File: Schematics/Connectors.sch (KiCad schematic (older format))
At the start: 130 parts, among them P501 CONN_02X05, P502 CONN_02X05, P503 CONN_02X05, P504 CONN_02X05, P505 CONN_6X2, P506 CONN_02X20, P507 CONN_02X05, P508 CONN_02X05, P509 CONN_02X05, P510 CONN_02X05, P511 CONN_02X05, P512 CONN_02X05, P513 CONN_02X05, P514 CONN_02X05, P515 CONN_02X05, P516 CONN_02X05, U501 NB3L553, U502 NB3L553

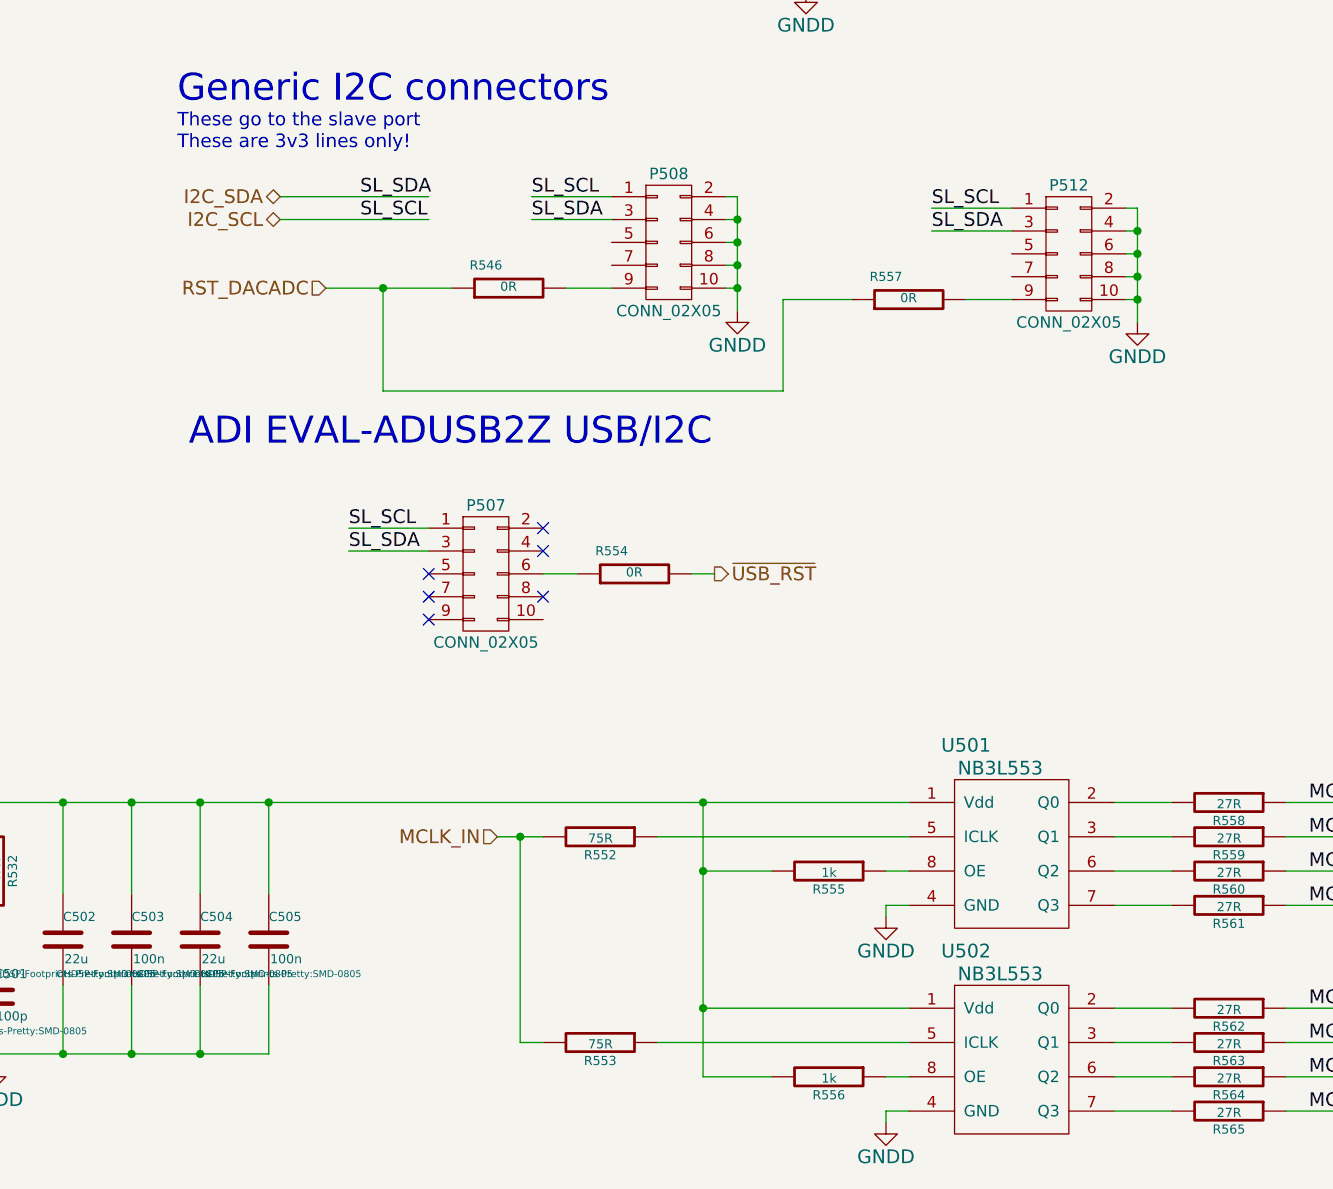
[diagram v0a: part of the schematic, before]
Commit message: WIP
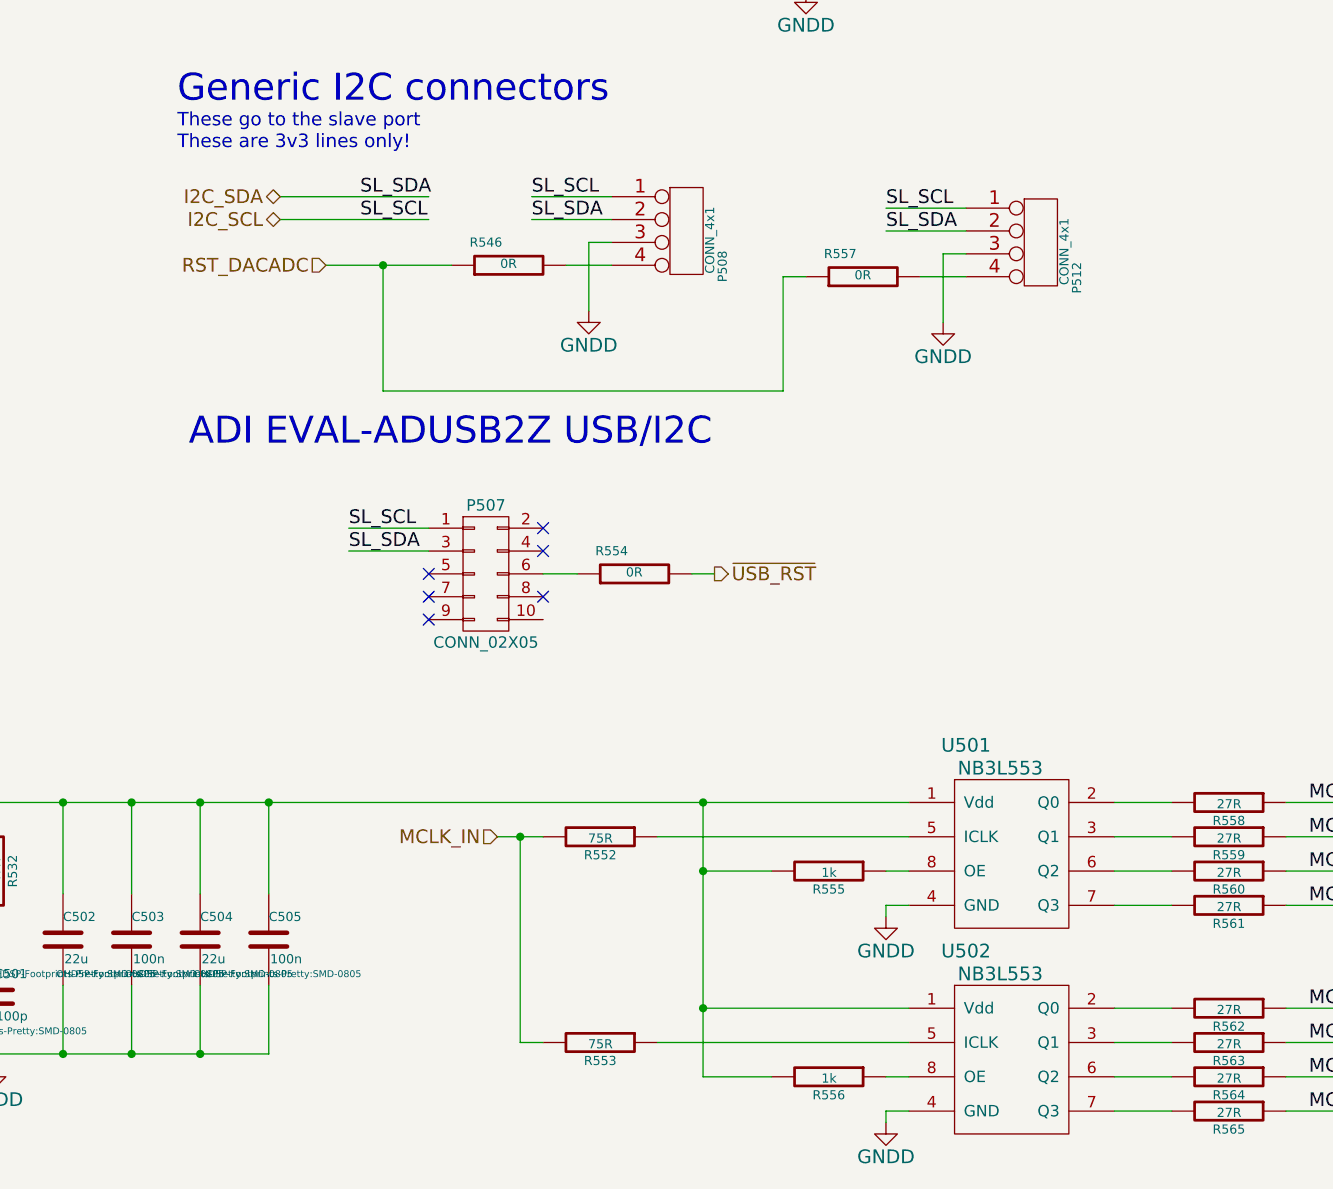
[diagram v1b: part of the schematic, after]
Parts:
- removed P508, P512: CONN_02X05, OHDSP-Footprints-Pretty:CONN_DIL_2X5, symbol CONN_02X05
- added P508, P512: CONN_4x1, OHDSP-Footprints-Pretty:CONN_SIL_4, symbol CONN_4x1
- P507: footprint OHDSP-Footprints-Pretty:CONN_DIL_2X5 -> OHDSP-Footprints-Pretty:CONN_DIL_2X5_BOX
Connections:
- wire segments 465 -> 457
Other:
- moved on the sheet: R546, R557
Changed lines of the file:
@@
 	1    0    0    -1
 $EndComp
-$Comp
-L CONN_02X05 P507
-U 1 1 54DC056C
-P 7400 8550
-F 0 "P507" H 7400 8850 50  0000 C CNN
-F 1 "CONN_02X05" H 7400 8250 50  0000 C CNN
-F 2 "OHDSP-Footprints-Pretty:CONN_DIL_2X5" H 7400 7350 60  0001 C CNN
-F 3 "" H 7400 7350 60  0000 C CNN
-	1    7400 8550
-	1    0    0    -1
-$EndComp
 Text Notes 6100 8000 0    118  ~ 0
 ADI EVAL-ADUSB2Z USB/I2C
@@
 L GNDD #PWR091
 U 1 1 54DC2149
-P 8500 7400
-F 0 "#PWR091" H 8500 7150 60  0001 C CNN
-F 1 "GNDD" H 8500 7250 60  0000 C CNN
-F 2 "" H 8500 7400 60  0000 C CNN
-F 3 "" H 8500 7400 60  0000 C CNN
-	1    8500 7400
+P 7850 7400
+F 0 "#PWR091" H 7850 7150 60  0001 C CNN
+F 1 "GNDD" H 7850 7250 60  0000 C CNN
+F 2 "" H 7850 7400 60  0000 C CNN
+F 3 "" H 7850 7400 60  0000 C CNN
+	1    7850 7400
 	1    0    0    -1
 $EndComp
@@
 $EndComp
 $Comp
-L CONN_02X05 P508
-U 1 1 54E480C2
-P 8200 7100
-F 0 "P508" H 8200 7400 50  0000 C CNN
-F 1 "CONN_02X05" H 8200 6800 50  0000 C CNN
-F 2 "OHDSP-Footprints-Pretty:CONN_DIL_2X5" H 8200 5900 60  0001 C CNN
-F 3 "" H 8200 5900 60  0000 C CNN
-	1    8200 7100
-	1    0    0    -1
-$EndComp
-$Comp
 L R R538
 U 1 1 54E4AF9E
@@
 $EndComp
 $Comp
-L CONN_02X05 P512
-U 1 1 54E55D44
-P 9950 7150
-F 0 "P512" H 9950 7450 50  0000 C CNN
-F 1 "CONN_02X05" H 9950 6850 50  0000 C CNN
-F 2 "OHDSP-Footprints-Pretty:CONN_DIL_2X5" H 9950 5950 60  0001 C CNN
-F 3 "" H 9950 5950 60  0000 C CNN
-	1    9950 7150
-	1    0    0    -1
-$EndComp
-$Comp
 L DIODE D501
 U 1 1 54E4E268
@@
 Text Label 7600 7000 0    60   ~ 0
 SL_SDA
-Text Label 9350 6950 0    60   ~ 0
-SL_SCL
-Text Label 9350 7050 0    60   ~ 0
-SL_SDA
-$Comp
-L GNDD #PWR0124
-U 1 1 551A75F1
-P 10250 7450
-F 0 "#PWR0124" H 10250 7200 60  0001 C CNN
-F 1 "GNDD" H 10250 7300 60  0000 C CNN
-F 2 "" H 10250 7450 60  0000 C CNN
-F 3 "" H 10250 7450 60  0000 C CNN
-	1    10250 7450
-	1    0    0    -1
-$EndComp
 $Comp
 L R R546
 U 1 1 551A97CD
-P 7500 7300
-F 0 "R546" V 7600 7400 40  0000 C CNN
-F 1 "0R" V 7507 7301 40  0000 C CNN
-F 2 "OHDSP-Footprints-Pretty:SMD-0805" V 7430 7300 30  0001 C CNN
-F 3 "~" H 7500 7300 30  0000 C CNN
-	1    7500 7300
+P 7500 7200
+F 0 "R546" V 7600 7300 40  0000 C CNN
+F 1 "0R" V 7507 7201 40  0000 C CNN
+F 2 "OHDSP-Footprints-Pretty:SMD-0805" V 7430 7200 30  0001 C CNN
+F 3 "~" H 7500 7200 30  0000 C CNN
+	1    7500 7200
 	0    -1   -1   0
 $EndComp
-Text HLabel 6700 7300 0    60   Input ~ 0
+Text HLabel 6700 7200 0    60   Input ~ 0
 RST_DACADC
 $Comp
 L R R557
 U 1 1 551B7A65
-P 9250 7350
-F 0 "R557" V 9350 7450 40  0000 C CNN
-F 1 "0R" V 9257 7351 40  0000 C CNN
-F 2 "OHDSP-Footprints-Pretty:SMD-0805" V 9180 7350 30  0001 C CNN
-F 3 "~" H 9250 7350 30  0000 C CNN
-	1    9250 7350
+P 9050 7250
+F 0 "R557" V 9150 7350 40  0000 C CNN
+F 1 "0R" V 9057 7251 40  0000 C CNN
+F 2 "OHDSP-Footprints-Pretty:SMD-0805" V 8980 7250 30  0001 C CNN
+F 3 "~" H 9050 7250 30  0000 C CNN
+	1    9050 7250
 	0    -1   -1   0
 $EndComp
@@
 $EndComp
 $Comp
-L GNDD #PWR0125
+L GNDD #PWR0124
 U 1 1 55623365
 P 9150 10050
-F 0 "#PWR0125" H 9150 9800 60  0001 C CNN
+F 0 "#PWR0124" H 9150 9800 60  0001 C CNN
 F 1 "GNDD" H 9150 9900 60  0000 C CNN
 F 2 "" H 9150 10050 60  0000 C CNN
@@
 $EndComp
 $Comp
-L GNDD #PWR0126
+L GNDD #PWR0125
 U 1 1 5562338E
 P 5250 10700
-F 0 "#PWR0126" H 5250 10450 60  0001 C CNN
+F 0 "#PWR0125" H 5250 10450 60  0001 C CNN
 F 1 "GNDD" H 5250 10550 60  0000 C CNN
 F 2 "" H 5250 10700 60  0000 C CNN
@@
 $EndComp
 $Comp
-L VPP #PWR0127
+L VPP #PWR0126
 U 1 1 556233B2
 P 4400 9400
-F 0 "#PWR0127" H 4400 9250 60  0001 C CNN
+F 0 "#PWR0126" H 4400 9250 60  0001 C CNN
 F 1 "VPP" H 4400 9550 60  0000 C CNN
 F 2 "" H 4400 9400 60  0000 C CNN
@@
 $EndComp
 $Comp
-L GNDD #PWR0128
+L GNDD #PWR0127
 U 1 1 5562ABC4
 P 9150 10950
-F 0 "#PWR0128" H 9150 10700 60  0001 C CNN
+F 0 "#PWR0127" H 9150 10700 60  0001 C CNN
 F 1 "GNDD" H 9150 10800 60  0000 C CNN
 F 2 "" H 9150 10950 60  0000 C CNN
@@
 $EndComp
 $Comp
-L GNDD #PWR0129
+L GNDD #PWR0128
 U 1 1 54E3DFB4
 P 13400 6700
-F 0 "#PWR0129" H 13400 6450 60  0001 C CNN
+F 0 "#PWR0128" H 13400 6450 60  0001 C CNN
 F 1 "GNDD" H 13400 6550 60  0000 C CNN
 F 2 "" H 13400 6700 60  0000 C CNN
@@
 Wire Wire Line
 	6800 8350 7150 8350
-Wire Wire Line
-	8500 7300 8450 7300
-Wire Wire Line
-	8500 6900 8500 7400
 Connection ~ 6200 5000
 Wire Wire Line
@@
 	7600 6900 7950 6900
 Wire Wire Line
-	9350 7050 9700 7050
-Wire Wire Line
-	9350 6950 9700 6950
-Wire Wire Line
-	10250 7350 10200 7350
-Wire Wire Line
-	10250 6950 10250 7450
-Wire Wire Line
-	10200 6950 10250 6950
-Connection ~ 10250 7350
-Wire Wire Line
-	10200 7050 10250 7050
-Connection ~ 10250 7050
-Wire Wire Line
-	10200 7250 10250 7250
-Connection ~ 10250 7250
-Wire Wire Line
-	8450 7200 8500 7200
-Connection ~ 8500 7300
+	6700 7200 7250 7200
 Wire Wire Line
-	8450 7000 8500 7000
-Connection ~ 8500 7200
+	8800 7250 8700 7250
+Connection ~ 6950 7200
 Wire Wire Line
-	8450 6900 8500 6900
-Connection ~ 8500 7000
-Wire Wire Line
-	7750 7300 7950 7300
-Wire Wire Line
-	6700 7300 7250 7300
-Wire Wire Line
-	8450 7100 8500 7100
-Connection ~ 8500 7100
-Wire Wire Line
-	10200 7150 10250 7150
-Connection ~ 10250 7150
-Wire Wire Line
-	9500 7350 9700 7350
-Wire Wire Line
-	9000 7350 8700 7350
-Connection ~ 6950 7300
-Wire Wire Line
-	6950 7300 6950 7750
+	6950 7200 6950 7750
 Wire Wire Line
 	6950 7750 8700 7750
 Wire Wire Line
-	8700 7750 8700 7350
+	8700 7750 8700 7250
 Wire Wire Line
 	8150 9700 9250 9700
@@
 Connection ~ 8350 9550
 Wire Wire Line
-	7650 9700 7450 9700
+	7450 9700 7650 9700
 Wire Wire Line
 	6150 10650 6150 10350
@@
 	6150 9550 6150 9950
 Wire Wire Line
-	8350 10750 8350 9550
+	8350 9550 8350 10750
+$Comp
+L CONN_02X05 P507
+U 1 1 54DC056C
+P 7400 8550
+F 0 "P507" H 7400 8850 50  0000 C CNN
+F 1 "CONN_02X05" H 7400 8250 50  0000 C CNN
+F 2 "OHDSP-Footprints-Pretty:CONN_DIL_2X5_BOX" H 7400 7350 60  0001 C CNN
+F 3 "" H 7400 7350 60  0000 C CNN
+	1    7400 8550
+	1    0    0    -1
+$EndComp
+$Comp
+L CONN_4x1 P508
+U 1 1 556C65A2
+P 7950 6900
+F 0 "P508" V 8435 6595 40  0000 C CNN
+F 1 "CONN_4x1" V 8380 6710 40  0000 C CNN
+F 2 "OHDSP-Footprints-Pretty:CONN_SIL_4" H 8290 6790 60  0001 C CNN
+F 3 "" H 8290 6790 60  0000 C CNN
+	1    7950 6900
+	1    0    0    -1
+$EndComp
+Wire Wire Line
+	7950 7100 7850 7100
+Wire Wire Line
+	7850 7100 7850 7400
+Wire Wire Line
+	7750 7200 7950 7200
+$Comp
+L GNDD #PWR0129
+U 1 1 556C820A
+P 9400 7450
+F 0 "#PWR0129" H 9400 7200 60  0001 C CNN
+F 1 "GNDD" H 9400 7300 60  0000 C CNN
+F 2 "" H 9400 7450 60  0000 C CNN
+F 3 "" H 9400 7450 60  0000 C CNN
+	1    9400 7450
+	1    0    0    -1
+$EndComp
+Text Label 9150 6950 0    60   ~ 0
+SL_SCL
+Text Label 9150 7050 0    60   ~ 0
+SL_SDA
+Wire Wire Line
+	9150 7050 9500 7050
+Wire Wire Line
+	9150 6950 9500 6950
+$Comp
+L CONN_4x1 P512
+U 1 1 556C821A
+P 9500 6950
+F 0 "P512" V 9985 6645 40  0000 C CNN
+F 1 "CONN_4x1" V 9930 6760 40  0000 C CNN
+F 2 "OHDSP-Footprints-Pretty:CONN_SIL_4" H 9840 6840 60  0001 C CNN
+F 3 "" H 9840 6840 60  0000 C CNN
+	1    9500 6950
+	1    0    0    -1
+$EndComp
+Wire Wire Line
+	9500 7150 9400 7150
+Wire Wire Line
+	9400 7150 9400 7450
+Wire Wire Line
+	9300 7250 9500 7250
 $EndSCHEMATC
